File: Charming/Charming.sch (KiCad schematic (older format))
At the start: 97 parts, among them SW1 SW_Push, SW10 SW_Push, SW11 SW_Push, SW12 SW_Push, SW13 SW_Push, SW14 SW_Push, SW15 SW_Push, SW16 SW_Push, SW17 SW_Push, SW18 SW_Push, SW19 SW_Push, SW2 SW_Push, SW20 SW_Push, SW21 SW_Push, SW22 SW_Push, SW23 SW_Push, SW24 SW_Push, SW25 SW_Push, SW26 SW_Push, SW27 SW_Push, SW28 SW_Push, SW29 SW_Push, SW3 SW_Push, SW30 SW_Push, SW31 SW_Push, SW32 SW_Push, SW33 SW_Push, SW34 SW_Push, SW35 SW_Push, SW36 SW_Push, SW37 SW_Push, SW38 SW_Push, SW39 SW_Push, SW4 SW_Push, SW40 SW_Push, SW41 SW_Push, SW42 SW_Push, SW43 SW_Push, SW44 SW_Push, SW45 SW_Push, SW46 SW_Push, SW47 SW_Push, SW48 SW_Push, SW5 SW_Push, SW6 SW_Push, SW7 SW_Push, SW8 SW_Push, SW9 SW_Push, U1 ProMicro

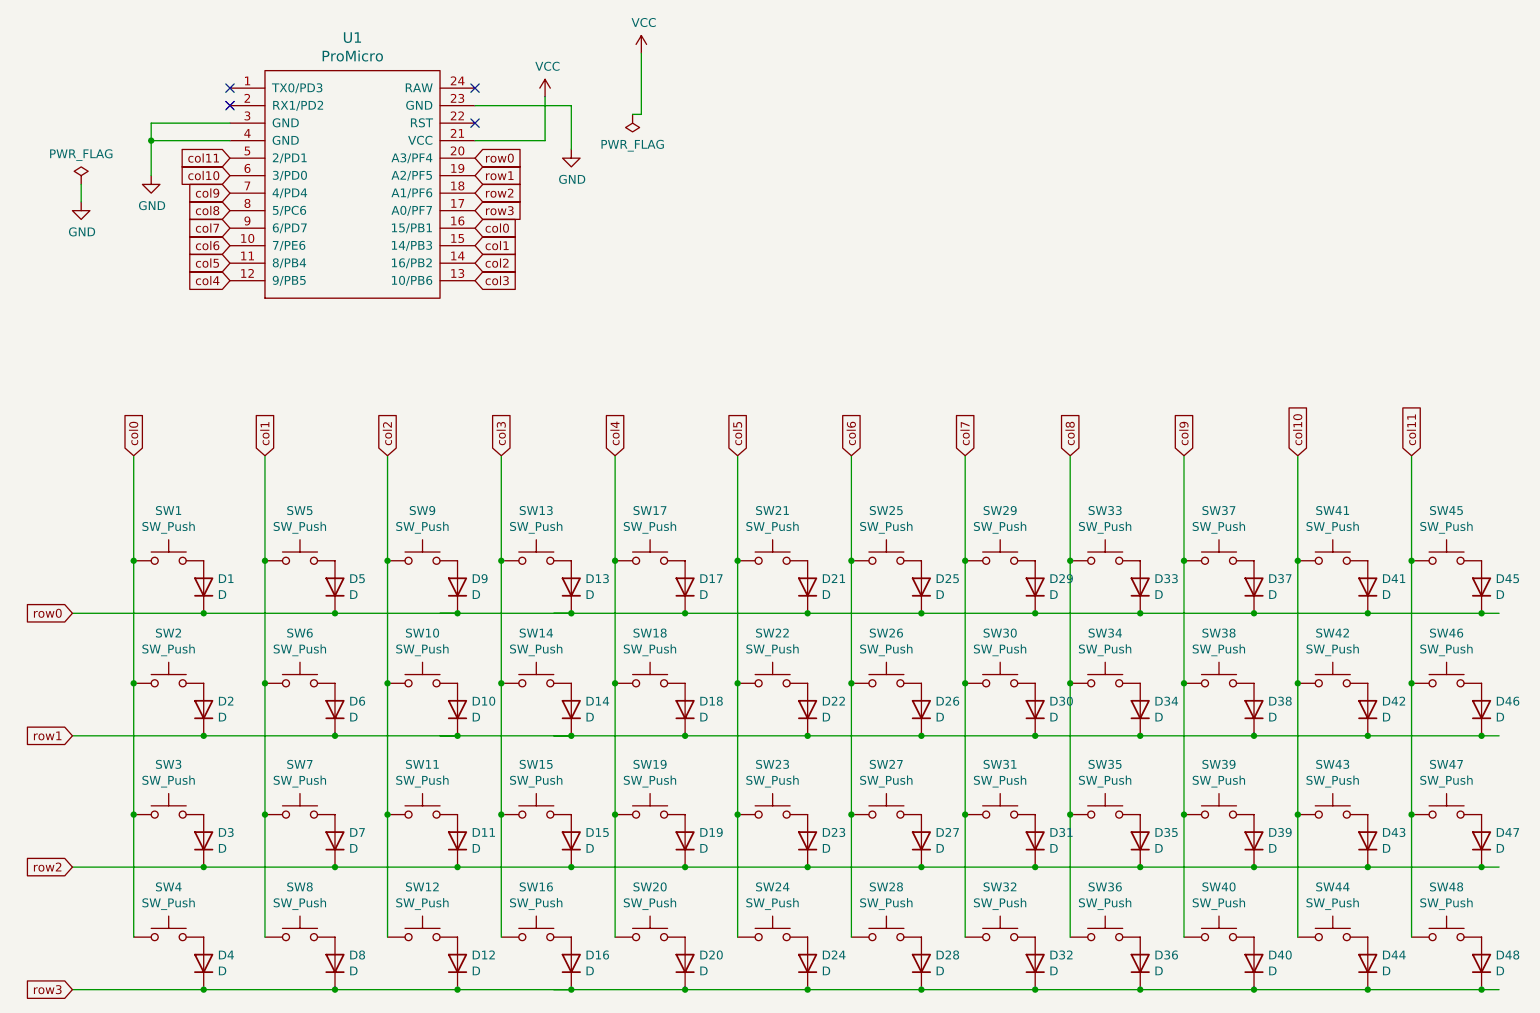
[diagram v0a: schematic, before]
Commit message: before row col changle
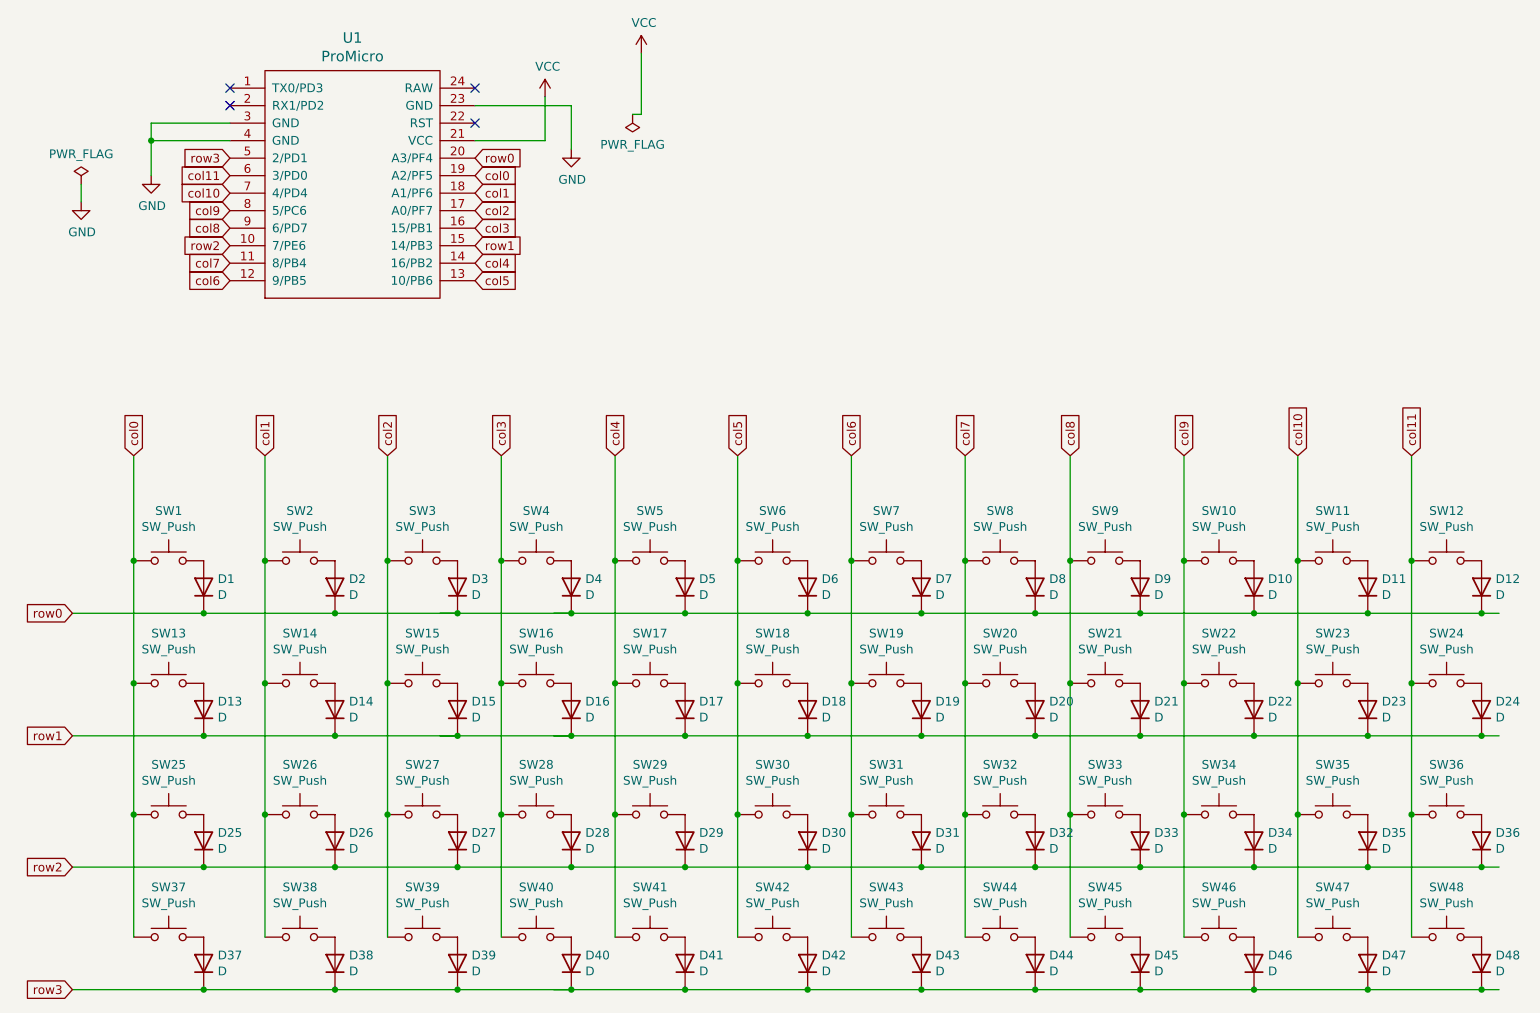
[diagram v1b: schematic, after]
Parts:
- renumbered D37 to D10, D41 to D11, D45 to D12, D2 to D13, D6 to D14, D10 to D15, D14 to D16, D18 to D17, D22 to D18, D26 to D19, D5 to D2, D30 to D20, D34 to D21, D38 to D22, D42 to D23, D46 to D24, D3 to D25, D7 to D26, D11 to D27, D15 to D28, D19 to D29, D9 to D3, D23 to D30, D27 to D31, D31 to D32, D35 to D33, D39 to D34, D43 to D35, D47 to D36, D4 to D37, D8 to D38, D12 to D39, D13 to D4, D16 to D40, D20 to D41, D24 to D42, D28 to D43, D32 to D44, D36 to D45, D40 to D46, D44 to D47, D17 to D5, D21 to D6, D25 to D7, D29 to D8, D33 to D9, SW37 to SW10, SW41 to SW11, SW45 to SW12, SW2 to SW13, SW6 to SW14, SW10 to SW15, SW14 to SW16, SW18 to SW17, SW22 to SW18, SW26 to SW19, SW5 to SW2, SW30 to SW20, SW34 to SW21, SW38 to SW22, SW42 to SW23, SW46 to SW24, SW3 to SW25, SW7 to SW26, SW11 to SW27, SW15 to SW28, SW19 to SW29, SW9 to SW3, SW23 to SW30, SW27 to SW31, SW31 to SW32, SW35 to SW33, SW39 to SW34, SW43 to SW35, SW47 to SW36, SW4 to SW37, SW8 to SW38, SW12 to SW39, SW13 to SW4, SW16 to SW40, SW20 to SW41, SW24 to SW42, SW28 to SW43, SW32 to SW44, SW36 to SW45, SW40 to SW46, SW44 to SW47, SW17 to SW5, SW21 to SW6, SW25 to SW7, SW29 to SW8, SW33 to SW9

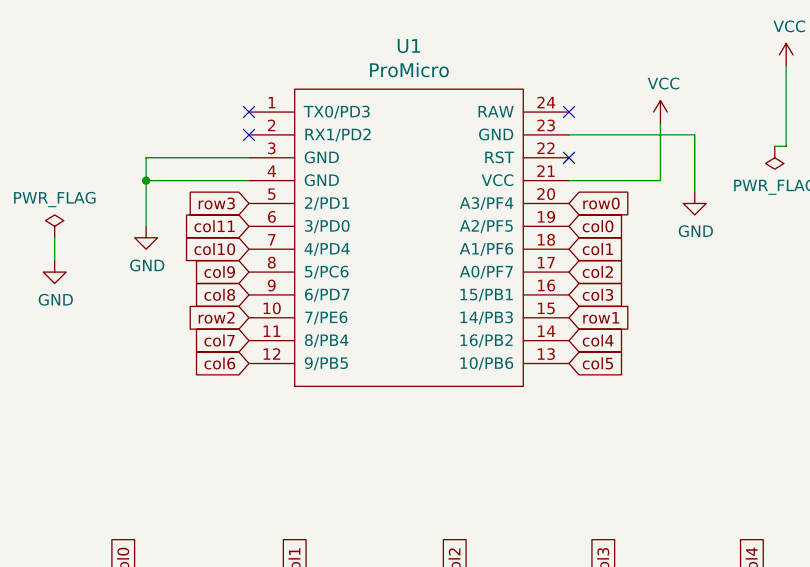
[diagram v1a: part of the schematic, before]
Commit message: v1
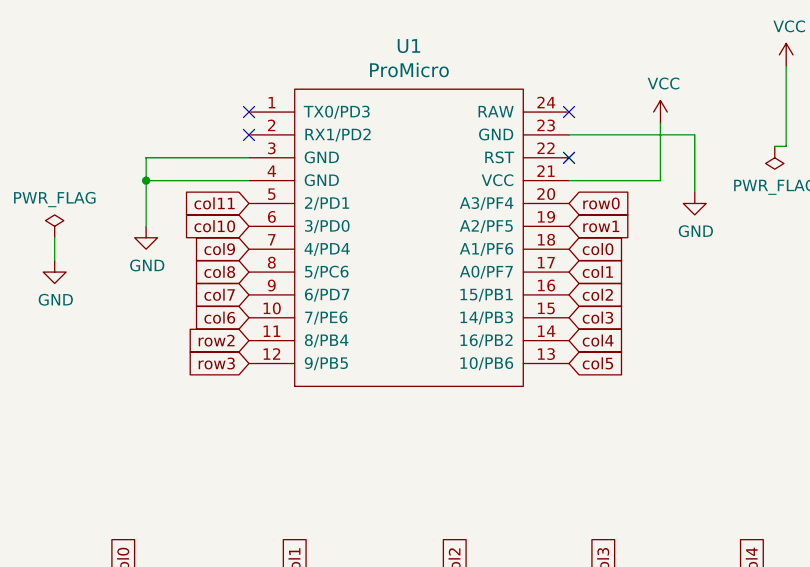
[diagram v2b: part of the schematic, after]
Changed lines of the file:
@@
 Wire Wire Line
 	3800 1200 4350 1200
+Text GLabel 3800 1800 2    50   Input ~ 0
+col1
+Text GLabel 3800 1600 2    50   Input ~ 0
+row1
 Text GLabel 3800 1700 2    50   Input ~ 0
-col1
+col0
+Text GLabel 2400 2200 0    50   Input ~ 0
+row3
+Text GLabel 3800 1900 2    50   Input ~ 0
+col2
 Text GLabel 3800 2000 2    50   Input ~ 0
-row1
-Text GLabel 3800 1600 2    50   Input ~ 0
-col0
-Text GLabel 2400 1500 0    50   Input ~ 0
-row3
-Text GLabel 3800 1800 2    50   Input ~ 0
-col2
-Text GLabel 3800 1900 2    50   Input ~ 0
 col3
 Text GLabel 3800 2100 2    50   Input ~ 0
@@
 Text GLabel 3800 2200 2    50   Input ~ 0
 col5
-Text GLabel 2400 2200 0    50   Input ~ 0
+Text GLabel 2400 2000 0    50   Input ~ 0
 col6
-Text GLabel 2400 2100 0    50   Input ~ 0
+Text GLabel 2400 1900 0    50   Input ~ 0
 col7
-Text GLabel 2400 1900 0    50   Input ~ 0
+Text GLabel 2400 1800 0    50   Input ~ 0
 col8
-Text GLabel 2400 1800 0    50   Input ~ 0
+Text GLabel 2400 1700 0    50   Input ~ 0
 col9
-Text GLabel 2400 1700 0    50   Input ~ 0
+Text GLabel 2400 1600 0    50   Input ~ 0
 col10
-Text GLabel 2400 1600 0    50   Input ~ 0
+Text GLabel 2400 1500 0    50   Input ~ 0
 col11
 NoConn ~ 3800 1300
@@
 	1    0    0    -1
 $EndComp
-Text GLabel 2400 2000 0    50   Input ~ 0
+Text GLabel 2400 2100 0    50   Input ~ 0
 row2
 $Comp
